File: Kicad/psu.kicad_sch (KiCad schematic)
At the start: 22 parts, among them J14 Conn_01x03_Pin, J15 Conn_01x03_Pin, J16 Conn_01x03_Pin, J17 Conn_01x03_Pin, J18 Conn_01x03_Pin, U15 L7912, U2 L7812, U3 XL1509-5.0

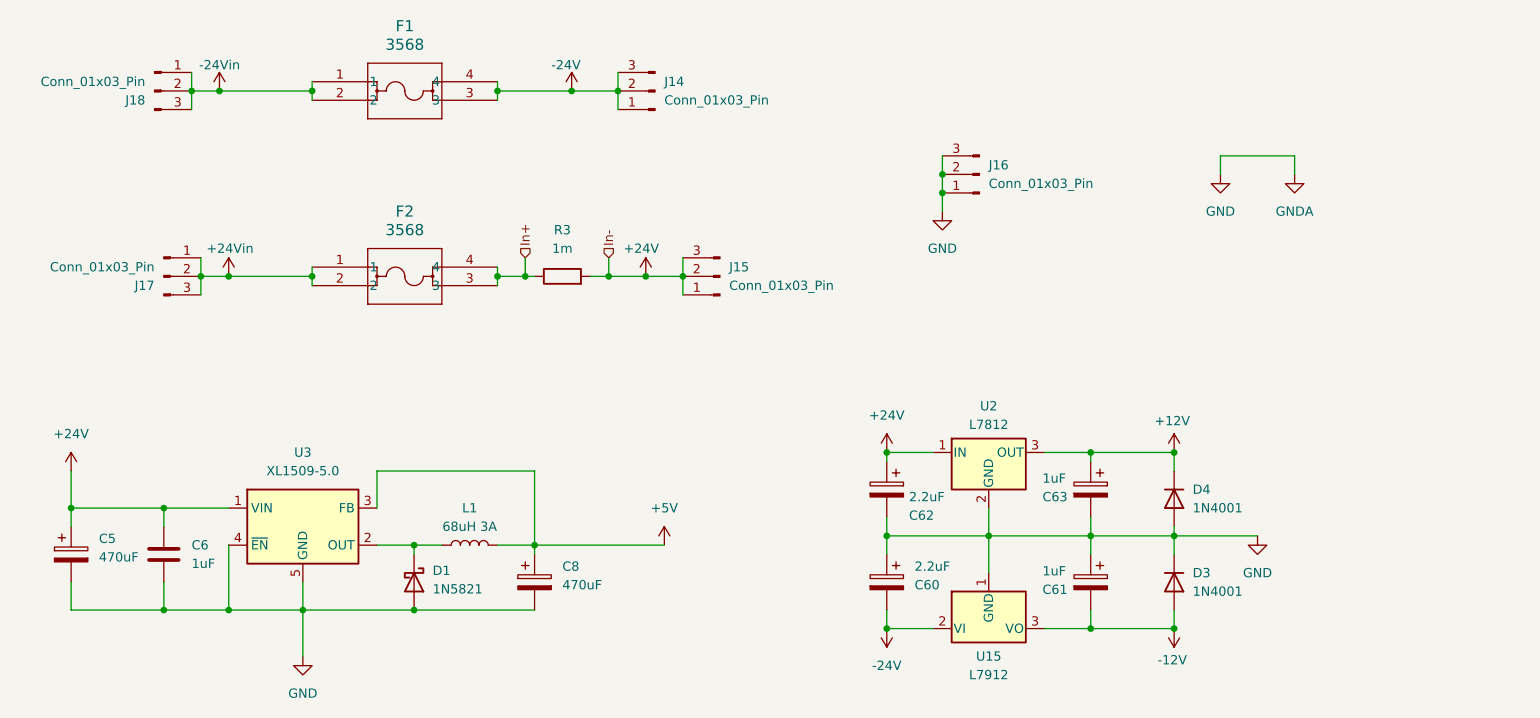
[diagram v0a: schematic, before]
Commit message: final schematic
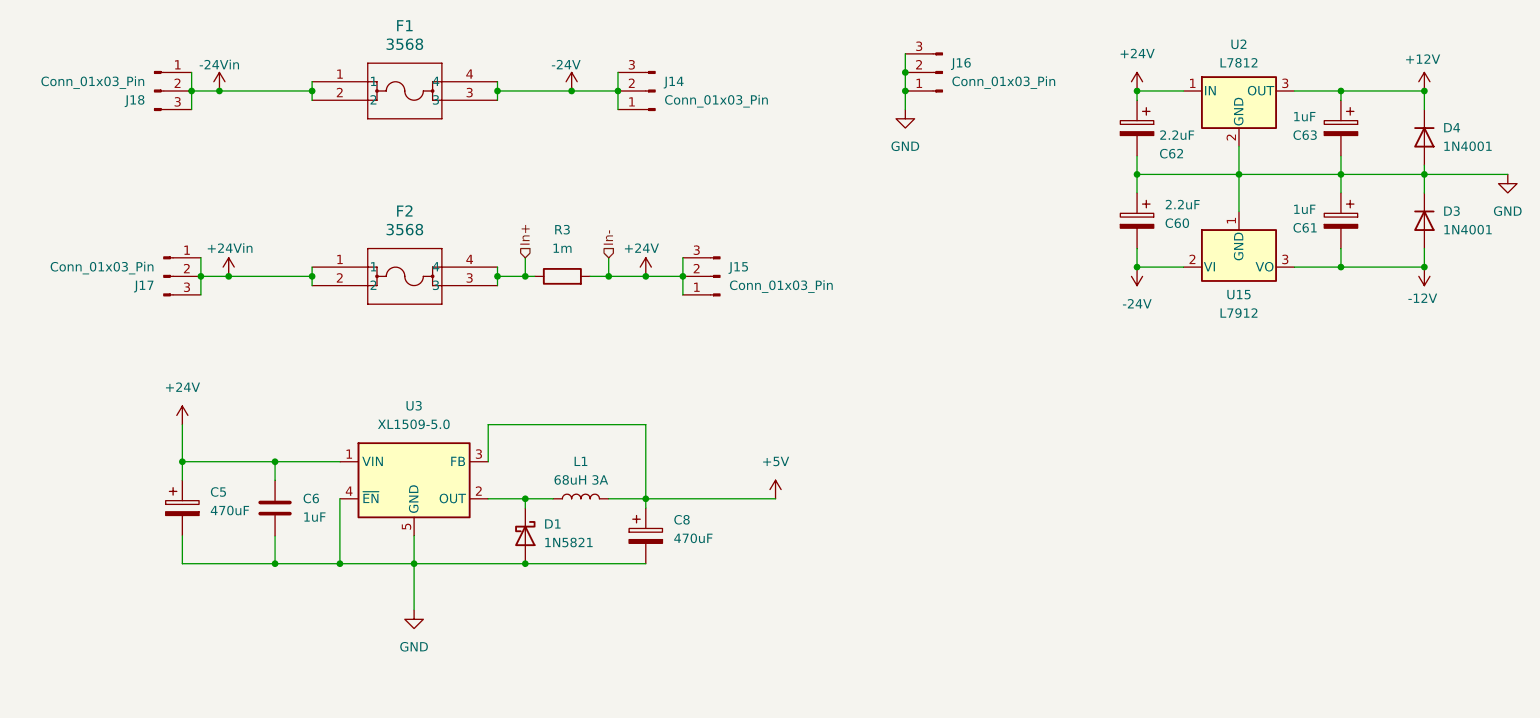
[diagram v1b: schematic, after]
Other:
- moved on the sheet: C5, C6, C60, C61, C62, C63, C8, D1, D3, D4, J16, L1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
